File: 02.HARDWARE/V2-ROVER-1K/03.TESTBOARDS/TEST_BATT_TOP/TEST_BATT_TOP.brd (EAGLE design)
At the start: 27 x 27 mm, 0 parts

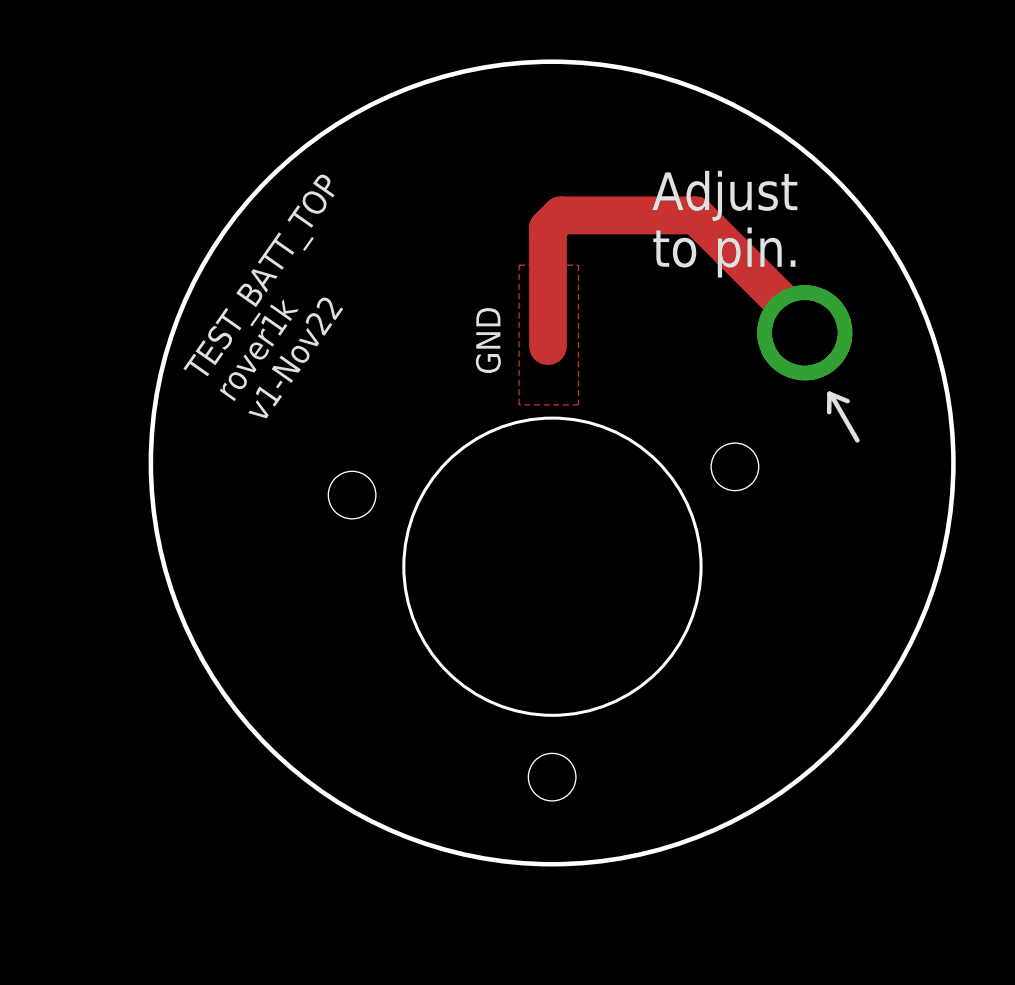
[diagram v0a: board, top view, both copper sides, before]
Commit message: Cierre ISSUE #3
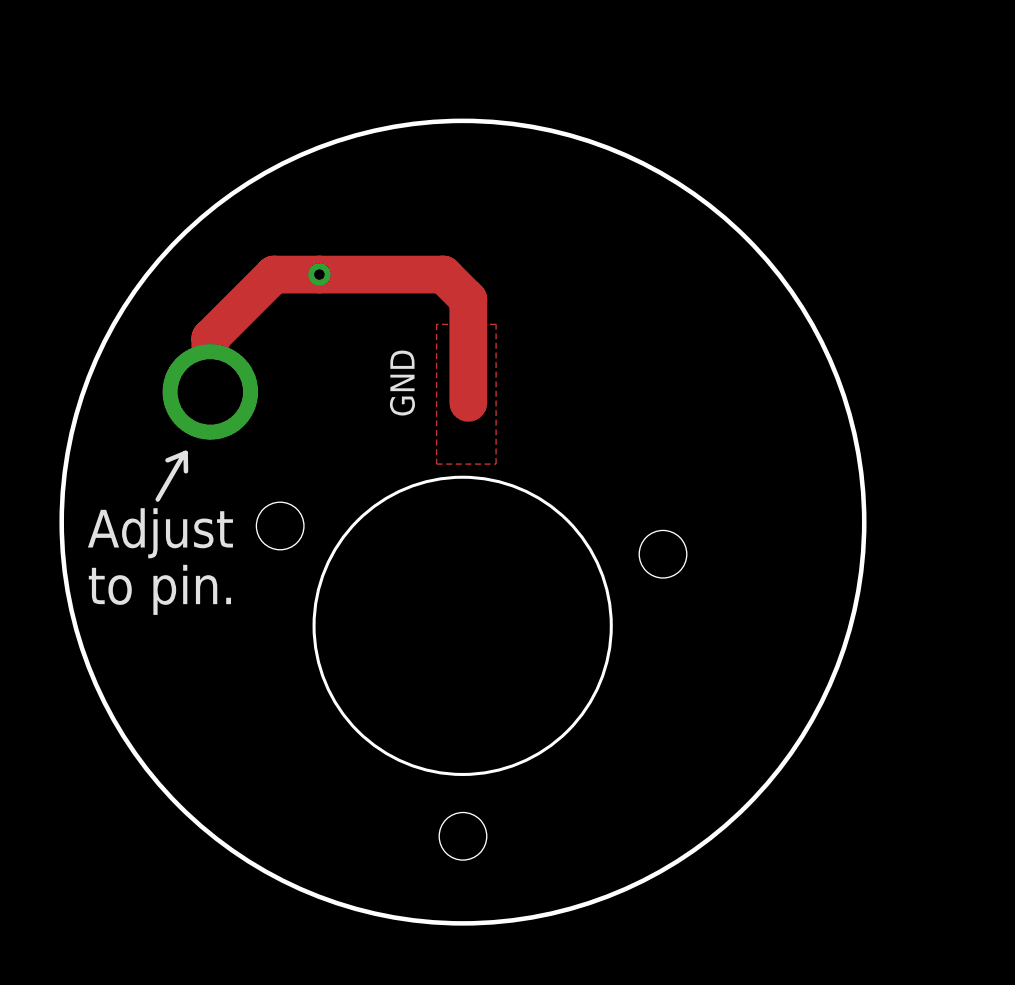
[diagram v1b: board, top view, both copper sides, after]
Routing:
- net N$1: track 0.00 -> 15.2 mm, vias 0 -> 2
- net GND: track 14.6 -> 0.00 mm, vias 1 -> 0
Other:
- board text added: "TEST_BATT_TOP rover1k v2-Nov22"
- board text removed: "TEST_BATT_TOP rover1k v1-Nov22"
